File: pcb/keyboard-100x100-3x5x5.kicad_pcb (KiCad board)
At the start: 2 copper layers, 95 x 94.2 mm, 126 parts, among them J1 Conn_01x04_Female, J2 Conn_01x04_Female, J3 Conn_01x05_Female, J4 Conn_01x05_Female, J5 Conn_01x05_Female, J6 Conn_01x05_Female, J7 Conn_01x05_Female, J8 Conn_01x05_Female, U1 BluePill_or_MiniF4_DIP40, U2 SN74LVC1T45DBV

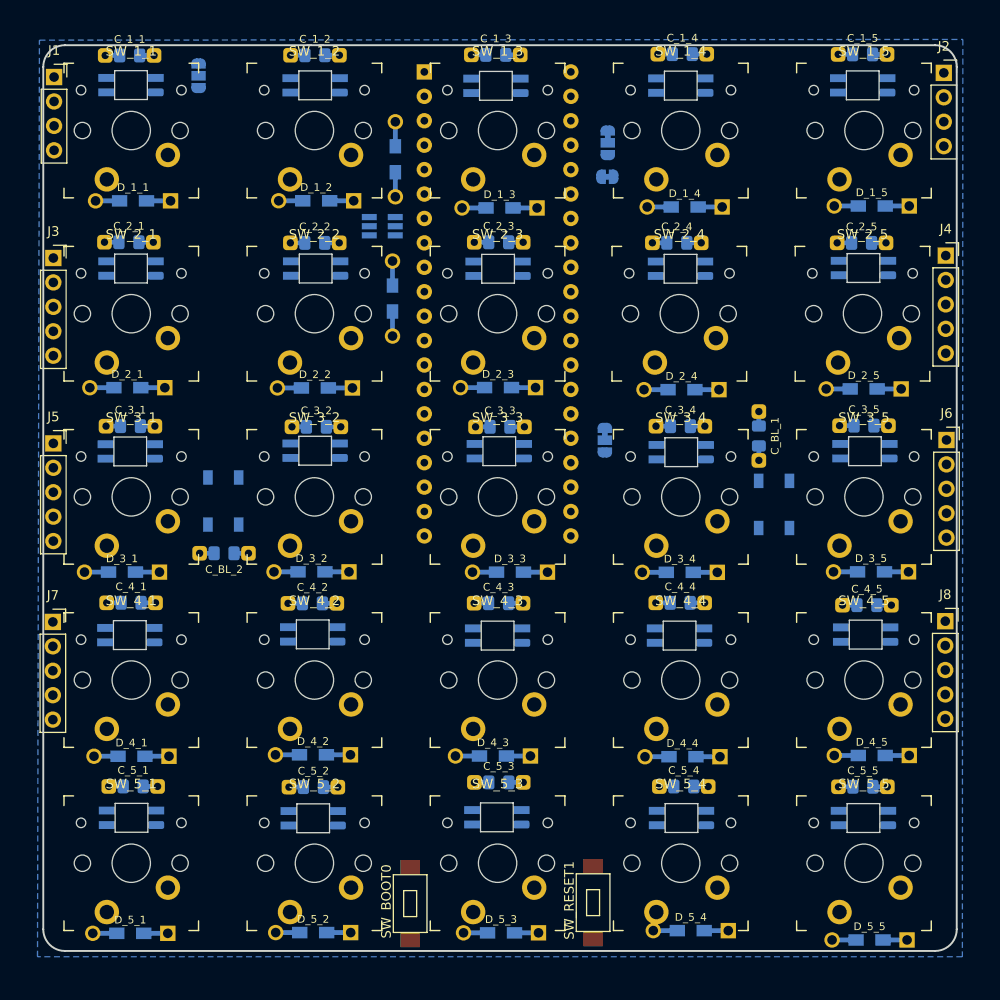
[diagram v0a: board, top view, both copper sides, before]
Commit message: WIP
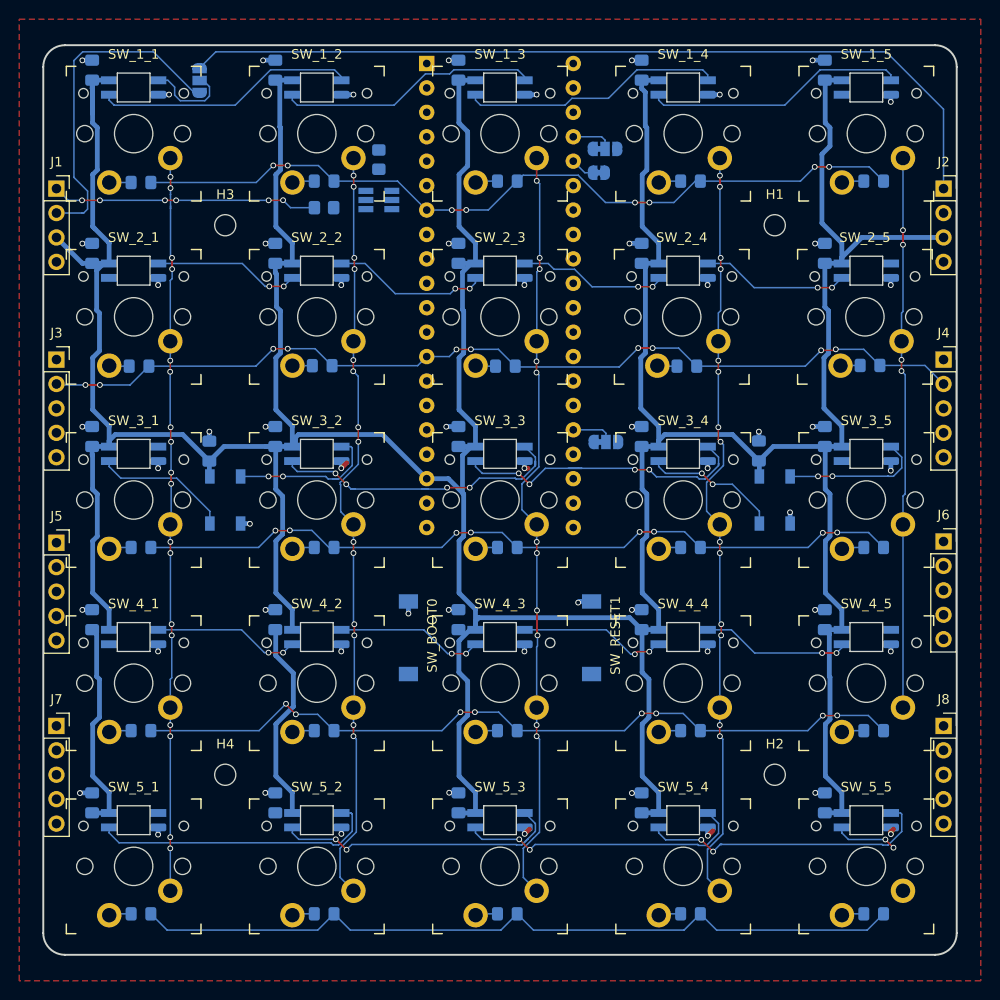
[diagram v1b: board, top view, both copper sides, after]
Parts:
- C_1_1, C_1_2, C_1_3, C_1_4, C_1_5, C_2_1, C_2_2, C_2_3, C_2_4, C_2_5, C_3_1, C_3_2, C_3_3, C_3_4, C_3_5, C_4_1, C_4_2, C_4_3, C_4_4, C_4_5, C_5_1, C_5_2, C_5_3, C_5_4, C_5_5: footprint ProjectLocal:C_0805_2012Metric_Pad1.18x1.45mm_HandSolder_Dual -> Capacitor_SMD:C_0805_2012Metric_Pad1.18x1.45mm_HandSolder
- C_BL_1: renamed from C_BL_2; footprint ProjectLocal:C_0805_2012Metric_Pad1.18x1.45mm_HandSolder_Dual -> Capacitor_SMD:C_0805_2012Metric_Pad1.18x1.45mm_HandSolder
- C_BL_2: renamed from C_BL_1; footprint ProjectLocal:C_0805_2012Metric_Pad1.18x1.45mm_HandSolder_Dual -> Capacitor_SMD:C_0805_2012Metric_Pad1.18x1.45mm_HandSolder
- D_1_1, D_1_2, D_1_3, D_1_4, D_1_5, D_2_1, D_2_2, D_2_3, D_2_4, D_2_5, D_3_1, D_3_2, D_3_3, D_3_4, D_3_5, D_4_1, D_4_2, D_4_3, D_4_4, D_4_5, D_5_1, D_5_2, D_5_3, D_5_4, D_5_5: footprint ProjectLocal:Diode-dual -> Diode_SMD:D_0805_2012Metric_Pad1.15x1.40mm_HandSolder
- H1, H2, H3, H4: footprint ProjectLocal:Bumpon_3M_F0502 -> MountingHole:MountingHole_2.2mm_M2
- R1, R2: footprint ProjectLocal:Resistor-Hybrid -> Resistor_SMD:R_0805_2012Metric_Pad1.20x1.40mm_HandSolder
- SW_BOOT0, SW_RESET1: moved to B.Cu
- moved SW_BOOT0 27.7 mm to (88.0, 115.4)
- moved SW_RESET1 27.5 mm to (107.0, 115.4)
- moved R1 14.5 mm to (84.9, 61.9)
- moved J2 12.0 mm to (143.6, 64.9)
- moved J1 11.6 mm to (51.4, 64.9)
- moved J8 10.9 mm to (143.6, 120.8)
- moved J7 10.8 mm to (51.4, 120.8)
- moved J4 10.8 mm to (143.6, 82.7)
- moved C_BL_1 10.7 mm to (67.3, 92.2), turned to 270 degrees
- moved J3 10.6 mm to (51.4, 82.7)
- moved J6 10.6 mm to (143.6, 101.6)
- moved J5 10.3 mm to (51.4, 101.7)
- moved R2 8.96 mm to (79.2, 66.9), turned to 180 degrees
- moved C_5_3 4.70 mm to (93.2, 128.8), turned to 270 degrees
- moved C_5_4 4.70 mm to (112.2, 128.8), turned to 270 degrees
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- renumbered LED_BL_2 to LED_BL_1, LED_BL_1 to LED_BL_2
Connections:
- J1 pad 1: /GND -> /RGB_DATA_START_OUT
- J1 pad 2: /5V -> /RGB_DATA_IN
- J1 pad 3: /RGB_DATA_IN -> /5V
- J1 pad 4: /RGB_DATA_START_OUT -> /GND
- J3 pad 1: /ROW5 -> /ROW1
- J3 pad 2: /ROW4 -> /ROW2
- J3 pad 4: /ROW2 -> /ROW4
- J3 pad 5: /ROW1 -> /ROW5
- J5 pad 1: /COL5 -> /COL1
- J5 pad 2: /COL4 -> /COL2
- J5 pad 4: /COL2 -> /COL4
- J5 pad 5: /COL1 -> /COL5
- J7 pad 1: /PREV_COL5 -> /PREV_COL1
- J7 pad 2: /PREV_COL4 -> /PREV_COL2
- J7 pad 4: /PREV_COL2 -> /PREV_COL4
- J7 pad 5: /PREV_COL1 -> /PREV_COL5
- LED_2_1 pad 2: Net-(LED_2_1-Pad2) -> /LED_3_IN
- LED_2_1 pad 4: /LED_2_IN -> Net-(LED_2_1-Pad4)
- LED_2_2 pad 2: Net-(LED_2_2-Pad2) -> Net-(LED_2_1-Pad4)
- LED_2_2 pad 4: Net-(LED_2_1-Pad2) -> Net-(LED_2_2-Pad4)
- LED_2_3 pad 2: Net-(LED_2_3-Pad2) -> Net-(LED_2_2-Pad4)
- LED_2_3 pad 4: Net-(LED_2_2-Pad2) -> Net-(LED_2_3-Pad4)
- LED_2_4 pad 2: Net-(LED_2_4-Pad2) -> Net-(LED_2_3-Pad4)
- LED_2_4 pad 4: Net-(LED_2_3-Pad2) -> Net-(LED_2_4-Pad4)
- LED_2_5 pad 2: /LED_3_IN -> Net-(LED_2_4-Pad4)
- LED_2_5 pad 4: Net-(LED_2_4-Pad2) -> /LED_2_IN
- LED_3_2 pad 4: Net-(LED_3_1-Pad2) -> Net-(LED_3_2-Pad4)
- LED_3_5 pad 4: Net-(LED_3_4-Pad2) -> Net-(LED_3_5-Pad4)
- LED_4_1 pad 2: Net-(LED_4_1-Pad2) -> /LED_5_IN
- LED_4_1 pad 4: /LED_4_IN -> Net-(LED_4_1-Pad4)
- LED_4_2 pad 2: Net-(LED_4_2-Pad2) -> Net-(LED_4_1-Pad4)
- LED_4_2 pad 4: Net-(LED_4_1-Pad2) -> Net-(LED_4_2-Pad4)
- LED_4_3 pad 2: Net-(LED_4_3-Pad2) -> Net-(LED_4_2-Pad4)
- LED_4_3 pad 4: Net-(LED_4_2-Pad2) -> Net-(LED_4_3-Pad4)
- LED_4_4 pad 2: Net-(LED_4_4-Pad2) -> Net-(LED_4_3-Pad4)
- LED_4_4 pad 4: Net-(LED_4_3-Pad2) -> Net-(LED_4_4-Pad4)
- LED_4_5 pad 2: /LED_5_IN -> Net-(LED_4_4-Pad4)
- LED_4_5 pad 4: Net-(LED_4_4-Pad2) -> /LED_4_IN
- LED_5_5 pad 2: /LED_BL_IN -> /RGB_DATA_OUT
- LED_BL_1 pad 2: /RGB_DATA_OUT -> Net-(LED_3_2-Pad4)
- LED_BL_1 pad 4: Net-(LED_BL_1-Pad2) -> Net-(LED_3_1-Pad2)
- LED_BL_2 pad 2: Net-(LED_BL_1-Pad2) -> Net-(LED_3_5-Pad4)
- LED_BL_2 pad 4: /LED_BL_IN -> Net-(LED_3_4-Pad2)
- U1 pad 11: (no net) -> Net-(U1-Pad11)
- U1 pad 12: (no net) -> Net-(U1-Pad12)
- U1 pad 17: (no net) -> Net-(U1-Pad17)
- U1 pad 21: (no net) -> Net-(U1-Pad21)
- U1 pad 22: (no net) -> Net-(U1-Pad22)
- U1 pad 23: (no net) -> Net-(U1-Pad23)
- U1 pad 24: (no net) -> Net-(U1-Pad24)
- U1 pad 40: (no net) -> /GND_or_5V
- U1 pad 6: (no net) -> Net-(U1-Pad6)
- U1 pad 8: (no net) -> /USB_DN
- U1 pad 9: (no net) -> /USB_DP
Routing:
- net /5V: track 0.00 -> 551.5 mm
- net /ROW2: track 0.00 -> 99.9 mm, vias 0 -> 10
- net /RGB_DATA_START_IN: track 0.00 -> 88.8 mm
- net /ROW1: track 0.00 -> 83.7 mm, vias 0 -> 8
- net /ROW4: track 0.00 -> 83.0 mm, vias 0 -> 8
- net /ROW5: track 0.00 -> 81.8 mm
- net /ROW3: track 0.00 -> 81.6 mm, vias 0 -> 8
- net /COL3: track 0.00 -> 79.4 mm, vias 0 -> 11
- net /COL2: track 0.00 -> 79.4 mm, vias 0 -> 14
- net /COL4: track 0.00 -> 79.3 mm, vias 0 -> 14
- net /COL1: track 0.00 -> 76.9 mm, vias 0 -> 18
- net /GND: track 0.00 -> 58.1 mm, vias 0 -> 56
- net /COL5: track 0.00 -> 57.7 mm, vias 0 -> 4
- net /RGB_DATA_IN: track 0.00 -> 34.7 mm
- net Net-(LED_3_3-Pad2): track 0.00 -> 32.4 mm, vias 0 -> 4
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- added copper zone on F.Cu, net /GND
- removed copper zone on B.Cu, net /GND
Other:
- board size 95 x 94.2 mm -> 95 x 94.6 mm
